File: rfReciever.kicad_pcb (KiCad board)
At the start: 4 copper layers, 32.8 x 23.2 mm, 36 parts, among them P2 USB_C_Plug_USB2.0, SW1 RF_RESET, SW2 RF_RESET, U1 CP2102N-Axx-xQFN20, U2 USBLC6-2SC6, X1 DigiXBeeRX900Micro

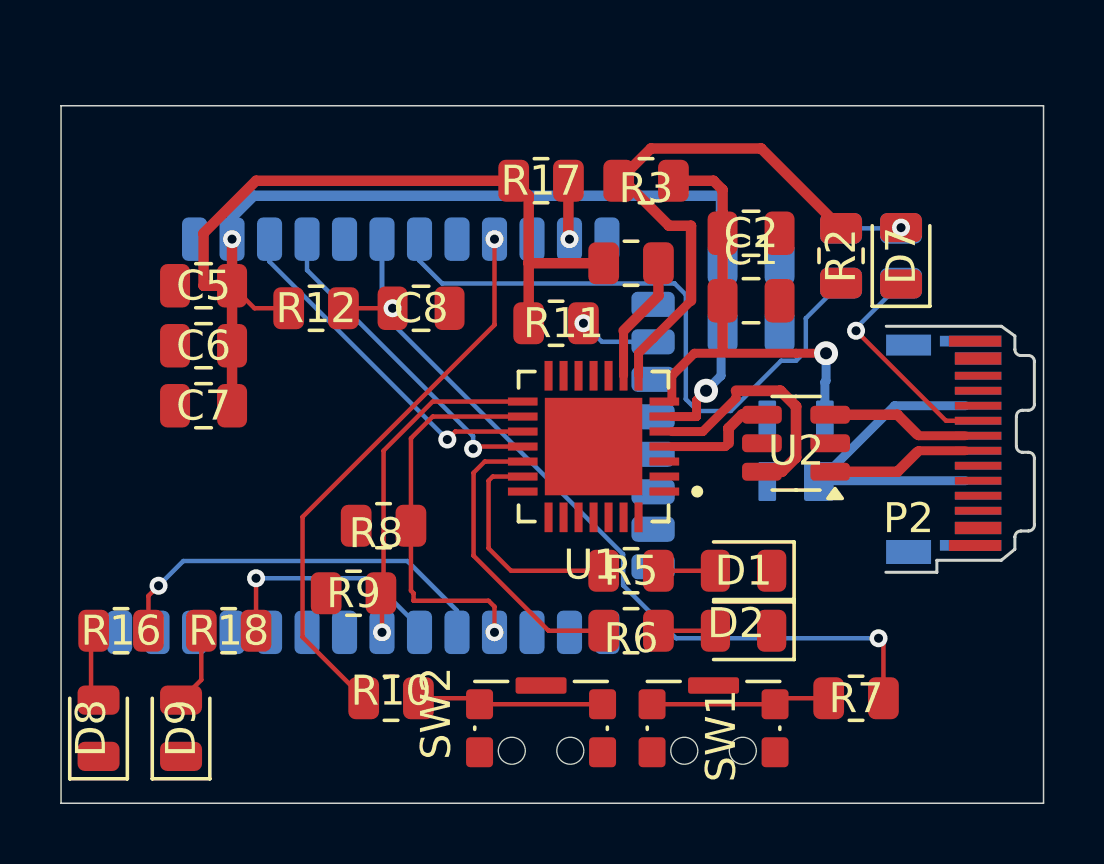
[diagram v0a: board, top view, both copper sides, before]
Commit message: Fixed up layout + shematic
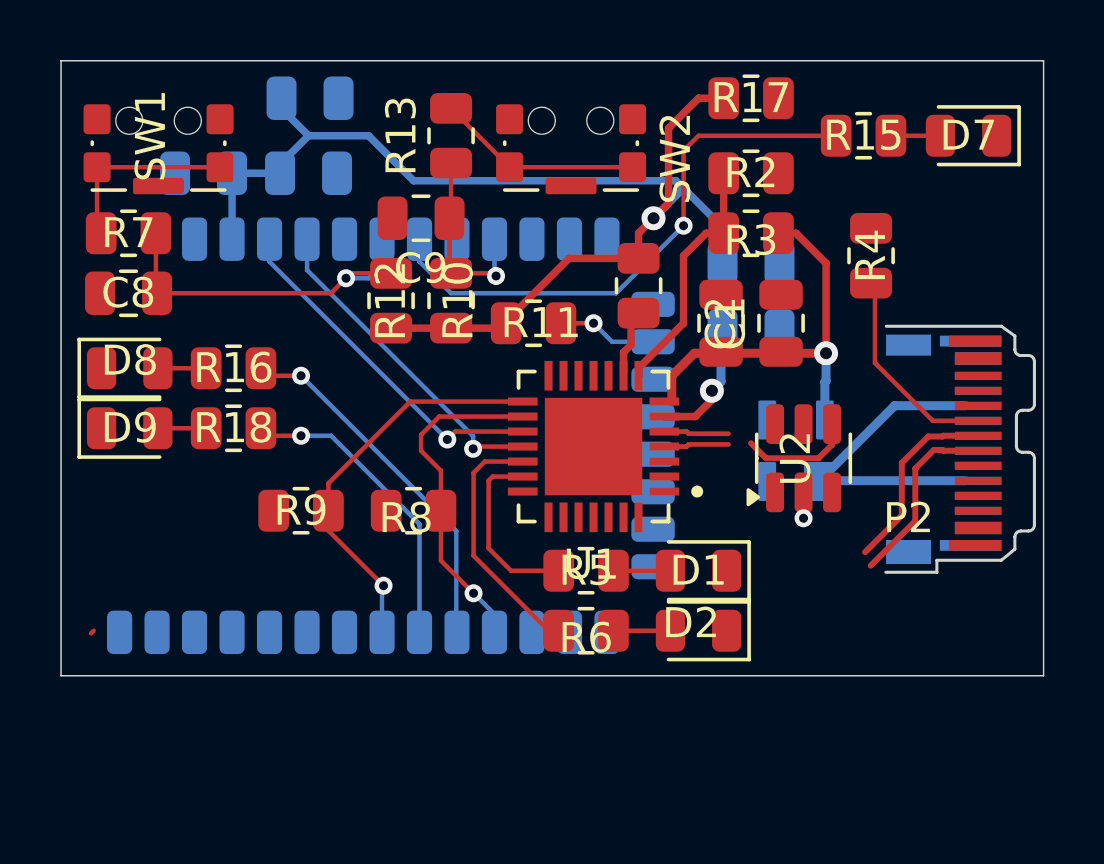
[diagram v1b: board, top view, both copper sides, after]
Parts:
- added C9: 1u, Capacitor_SMD:C_0805_2012Metric, F.Cu at (106.8, 65.8)
- added R13: 1k, Resistor_SMD:R_0805_2012Metric, F.Cu at (107.8, 63.0)
- C5, C6, C7: moved to B.Cu
- R15, R4: moved to F.Cu
- SW2: value RF_RESET -> RF_SLEEP
- moved R7 28.8 mm to (97.0, 66.2)
- moved SW1 26.9 mm to (98.0, 63.2), turned to 180 degrees
- moved SW2 19.5 mm to (111.8, 63.2), turned to 180 degrees
- moved R10 13.4 mm to (107.8, 68.5), turned to -90 degrees
- moved D8 12.0 mm to (97.0, 70.8), turned to 0 degrees
- moved C7 10.8 mm to (103.0, 61.8), turned to 0 degrees
- moved D9 10.1 mm to (97.0, 72.8), turned to 0 degrees
- moved C8 9.76 mm to (97.0, 68.2), turned to 180 degrees
- moved R16 9.52 mm to (100.5, 70.8)
- moved R17 7.52 mm to (117.8, 61.8)
- moved R18 6.75 mm to (100.5, 72.8)
- moved C6 6.73 mm to (103.0, 64.2), turned to 0 degrees
- moved D7 4.59 mm to (125.0, 63.0), turned to 180 degrees
- moved R15 4.07 mm to (121.5, 63.0), turned to 0 degrees
- moved R2 4.07 mm to (117.8, 64.2), turned to 0 degrees
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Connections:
- net /RF_SW_RSTO renamed /RF_SW_RESET
- D3 pad 1: Net-(D3-Pad1) -> +5V
- P2 pad A4: Net-(D3-Pad1) -> +5V
- P2 pad A9: Net-(D3-Pad1) -> +5V
- P2 pad B4: Net-(D3-Pad1) -> +5V
- P2 pad B9: Net-(D3-Pad1) -> +5V
- R10 pad 2: Net-(R10-Pad2) -> +3.3V
- SW2 pad 1: Net-(R10-Pad2) -> /RF_SW_SLEEP
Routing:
- net /RF_RESET: track 30.3 -> 12.6 mm, vias 2 -> 1
- net /RF_SLEEP: track 18.9 -> 6.50 mm
- net Net-(D3-Pad1): track 10.8 -> 0.00 mm
- net /BRIDGE_VBUS: track 17.7 -> 8.27 mm
- net +5V: track 15.5 -> 24.4 mm
- net +3.3V: track 55.4 -> 48.4 mm
- net /RF_SW_SLEEP: track 0.00 -> 6.87 mm
- net Net-(R10-Pad2): track 6.22 -> 0.00 mm
- net /USB_OUT_D-: track 8.10 -> 2.36 mm
- net /RF_PWM: track 21.3 -> 18.7 mm, vias 0 -> 1
- net /USB_OUT_D+: track 3.73 -> 5.95 mm
- net /RF_ASSOCIATE: track 8.04 -> 10.2 mm
- net /USB_IN_D+: track 4.80 -> 6.76 mm
- net /RF_BOOTMODE: track 1.96 -> 0.00 mm, vias 1 -> 0
- net /BRIDGE_3.3: track 4.23 -> 2.29 mm
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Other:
- board size 32.8 x 23.2 mm -> 32.8 x 20.5 mm
